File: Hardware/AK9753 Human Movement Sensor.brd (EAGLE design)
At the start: 25.4 x 25.4 mm, 30 parts, among them J2 Qwiic Right Angle, J3 PTH, J4 Qwiic Right Angle, U2 AK9753

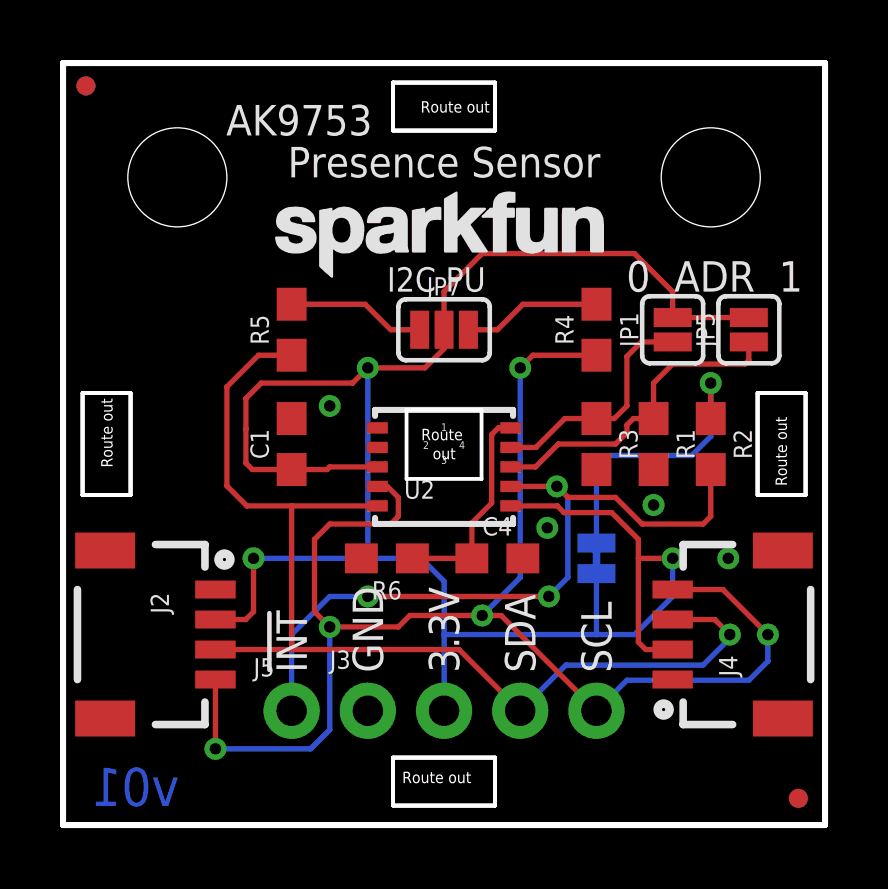
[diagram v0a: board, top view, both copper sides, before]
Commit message: Pre Review commit
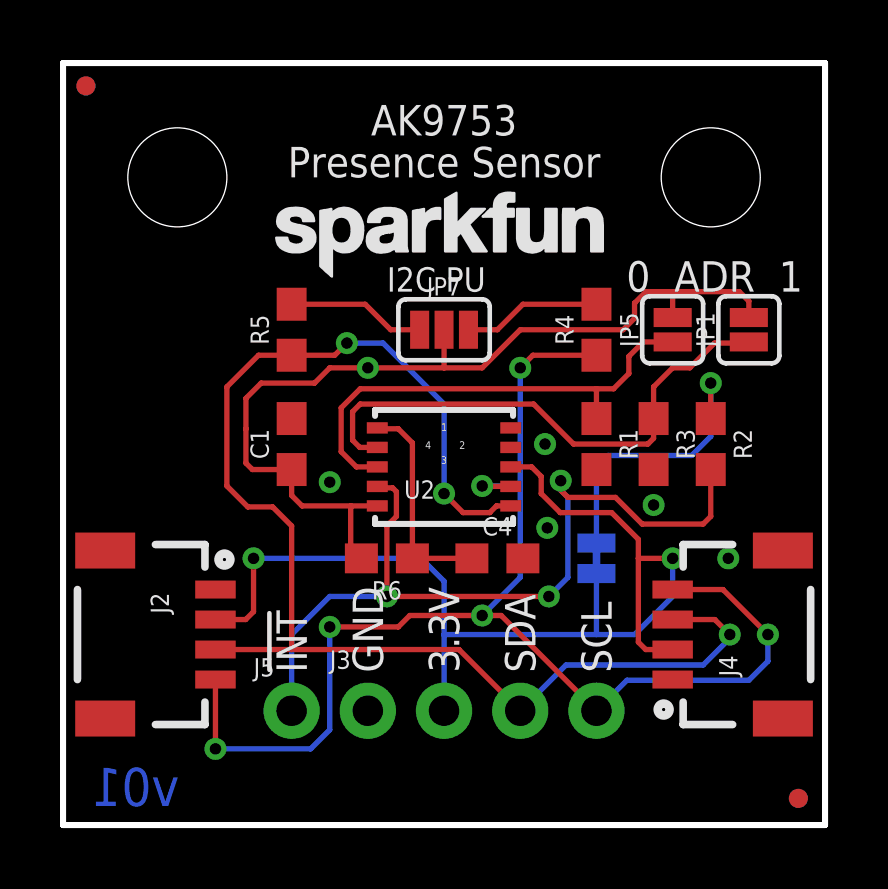
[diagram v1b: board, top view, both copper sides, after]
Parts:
- removed U$3: CWM 0.5 GI V1, openPIR-temp:LENS-CWM-0.5-GI-V1
- moved JP1 2.54 mm to (22.9, 16.5)
- moved JP5 2.54 mm to (20.3, 16.5)
- moved R1 1.90 mm to (17.8, 12.7)
- moved R3 1.90 mm to (19.7, 12.7)
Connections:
- net !INT: now also U2.7; no longer U2.4
- net 3.3V: now also U2.3, U2.6; no longer U2.5, U2.8
- net ADR0: now also U2.9; no longer U2.2
- net ADR1: now also U2.8; no longer U2.3
- net GND: now also U2.1, U2.2; no longer U2.10, U2.9
- net SCL: now also U2.4; no longer U2.7
- net SDA: now also U2.5; no longer U2.6
- net VDD: now also U2.10; no longer U2.1
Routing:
- net ADR0: track 7.82 -> 18.2 mm
- net SDA: track 37.2 -> 45.6 mm, vias 1 -> 3
- net SCL: track 50.5 -> 45.0 mm, vias 5 -> 6
- net ADR1: track 10.9 -> 16.2 mm
- net !INT: track 24.6 -> 27.6 mm
- net 3.3V: track 71.4 -> 69.6 mm
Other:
- board text removed: "Route"
- board text removed: "Route out"
- board text removed: "out"
